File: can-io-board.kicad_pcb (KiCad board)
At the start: 2 copper layers, 16.4 x 20.1 mm, 24 parts, among them J1 CONN_IO, J2 CONN_PWM, U1 STM32F302K8U6, U2 MCP1703, U3 MAX3051, X1 16MHz 10ppm

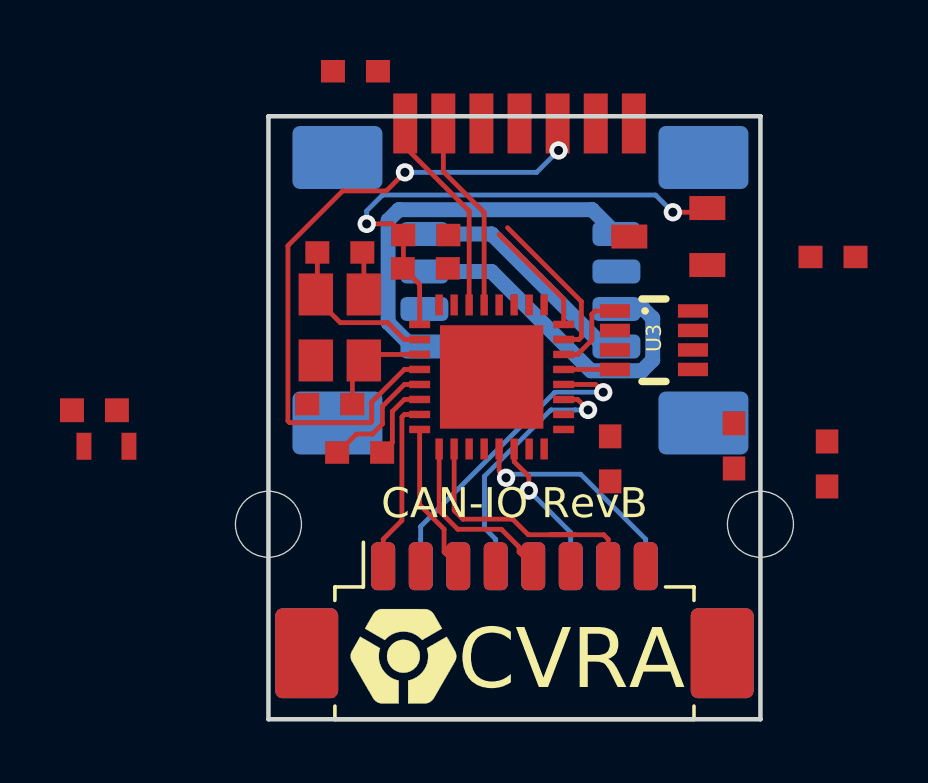
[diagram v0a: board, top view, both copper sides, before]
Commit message: Routing almost finished
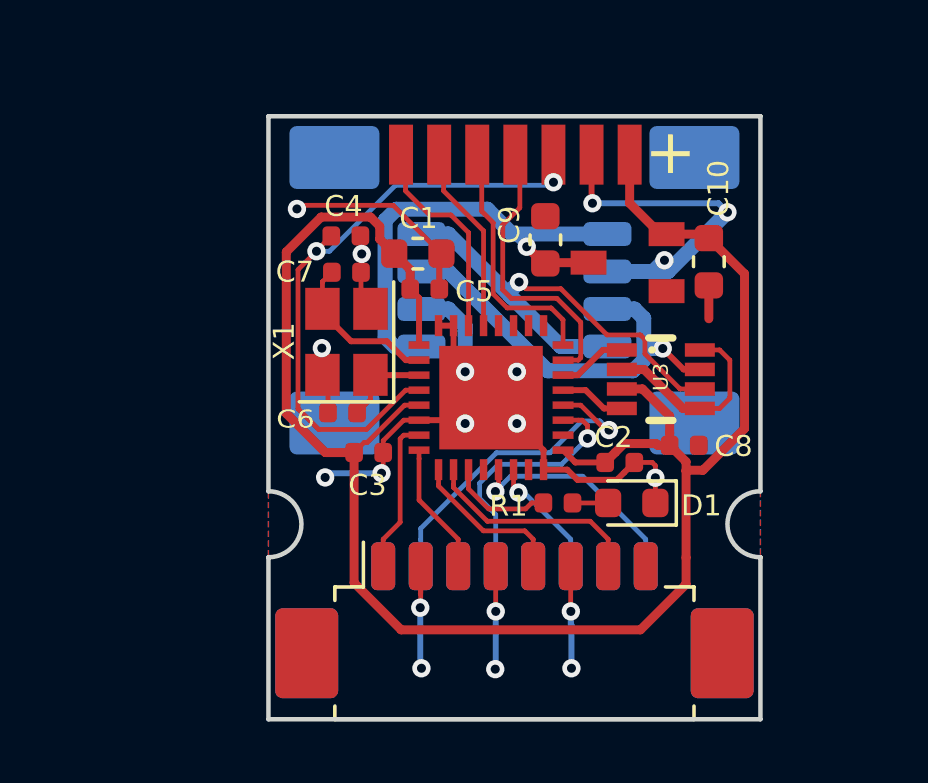
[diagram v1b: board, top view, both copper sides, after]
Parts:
- removed H1, H2: MountingHole M2, MountingHole:MountingHole_2.2mm_M2_DIN965
- C1, C10, C9: footprint Capacitors_SMD:C_0603 -> Capacitor_SMD:C_0603_1608Metric
- C2, C3, C4, C5, C6, C7, C8: footprint Capacitors_SMD:C_0603 -> Capacitor_SMD:C_0402_1005Metric
- D1: footprint LEDs:LED-0603 -> LED_SMD:LED_0603_1608Metric
- G***: moved to B.Cu
- R1: footprint Resistors_SMD:R_0603 -> Resistor_SMD:R_0402_1005Metric
- X1: footprint _div:_TSX-3225-SMD-XTAL -> Crystal:Crystal_SMD_SeikoEpson_TSX3225-4Pin_3.2x2.5mm
- moved D1 18.2 mm to (95.9, 77.1), turned to 180 degrees
- moved R1 15.2 mm to (93.5, 77.1)
- moved C9 12.0 mm to (93.0, 68.3), turned to 90 degrees
- moved G*** 9.18 mm to (92.2, 73.9), turned to 90 degrees
- moved C4 5.50 mm to (86.4, 68.2)
- moved C10 4.14 mm to (98.5, 69.0), turned to 270 degrees
- moved C8 1.66 mm to (97.7, 75.2), turned to 0 degrees
- moved U2 1.61 mm to (97.1, 70.0)
- moved U3 1.32 mm to (95.6, 72.0)
- moved CONN1 1.05 mm to (92.0, 65.5)
- moved C7 0.70 mm to (86.4, 69.4)
- moved C5 0.69 mm to (89.0, 70.0)
- moved U1 0.69 mm to (91.2, 73.6)
- moved C1 0.68 mm to (88.8, 68.8)
- moved X1 0.53 mm to (86.4, 71.7)
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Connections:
- D1 pad 1: Net-(D1-Pad1) -> GND
- D1 pad 2: /LED -> Net-(D1-Pad2)
- R1 pad 1: Net-(D1-Pad1) -> /LED
- R1 pad 2: GND -> Net-(D1-Pad2)
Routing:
- net GND: track 4.01 -> 61.9 mm, vias 0 -> 19
- net VCC: track 21.0 -> 61.8 mm, vias 2 -> 0
- net Net-(CONN2-Pad4): track 7.95 -> 16.2 mm, vias 0 -> 1
- net /SWCK: track 3.89 -> 7.72 mm
- net /SWIO: track 5.29 -> 8.99 mm
- net /LED: track 0.00 -> 3.50 mm
- net /5V_CAN: track 13.0 -> 16.1 mm, vias 0 -> 1
- net Net-(CONN2-Pad3): track 11.9 -> 13.8 mm, vias 0 -> 1
- net /IO3_PA3: track 9.30 -> 7.36 mm
- net Net-(D1-Pad2): track 0.00 -> 1.19 mm
- net /RST: track 22.0 -> 20.9 mm
- net /IO1_PA1: track 5.32 -> 4.41 mm
- net /IO_PB6_I2C1SCL_UART1TX: track 6.54 -> 5.64 mm
- net /IO2_PA2: track 6.06 -> 5.34 mm
- net /IO0_PA0: track 5.86 -> 5.16 mm
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- added copper zone on B.Cu, net GND
- added copper zone on F.Cu, net GND
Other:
- outline, holes or cut-outs redrawn
- board text added: "+"
- board text added: "Designed by: Michael Spieler"
